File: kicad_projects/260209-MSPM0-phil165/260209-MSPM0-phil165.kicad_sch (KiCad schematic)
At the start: 17 parts, among them J1 USB_C_Receptacle_USB2.0_16P, U1 MSPM0G3507SPTR, U2 USBLC6-2SC6, U3 SPX3819M5-L-3-3, X1 8MHz

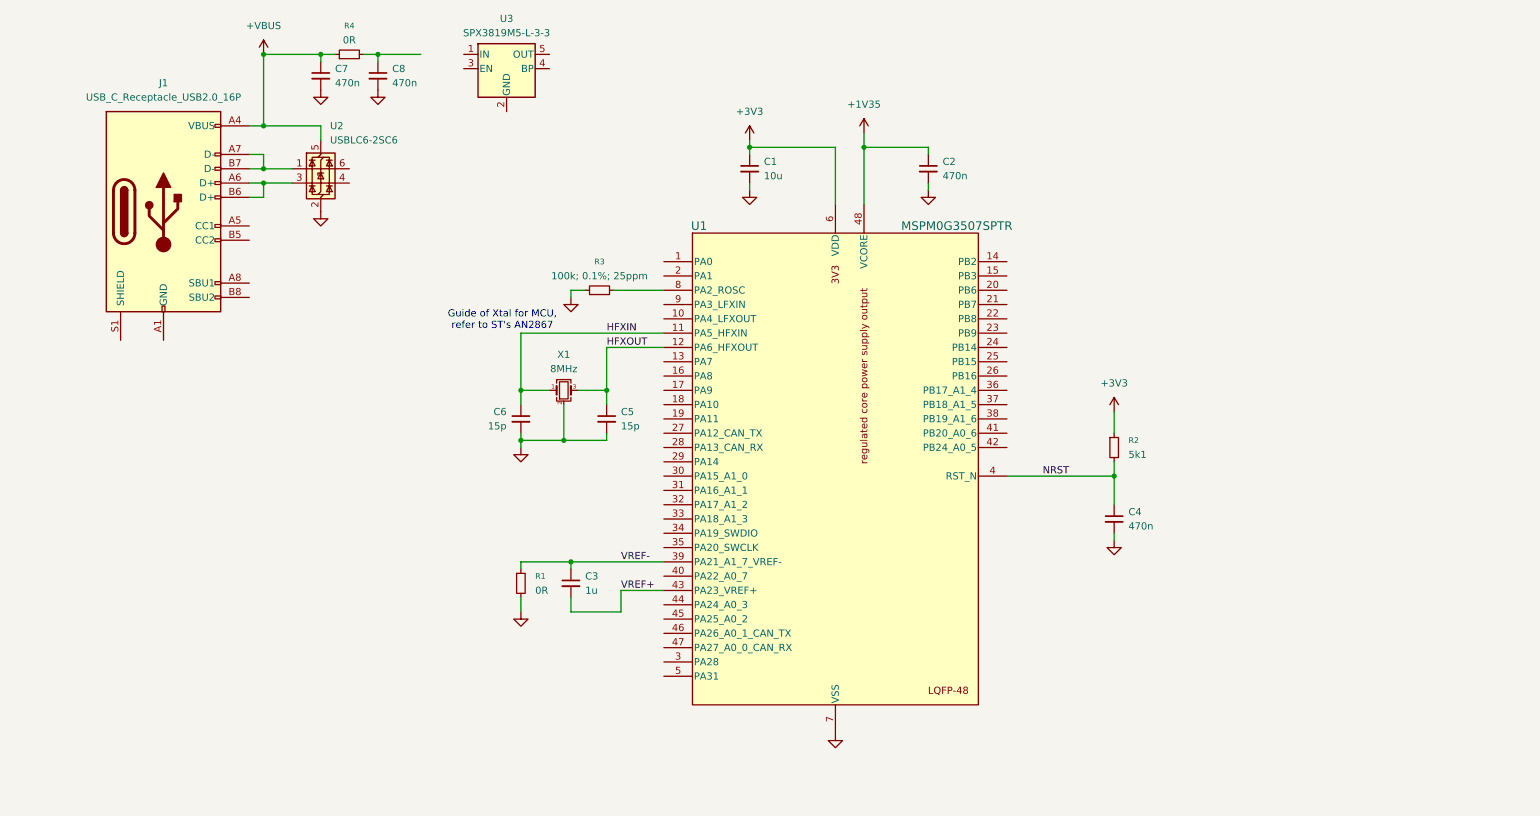
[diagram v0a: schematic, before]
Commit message: regular
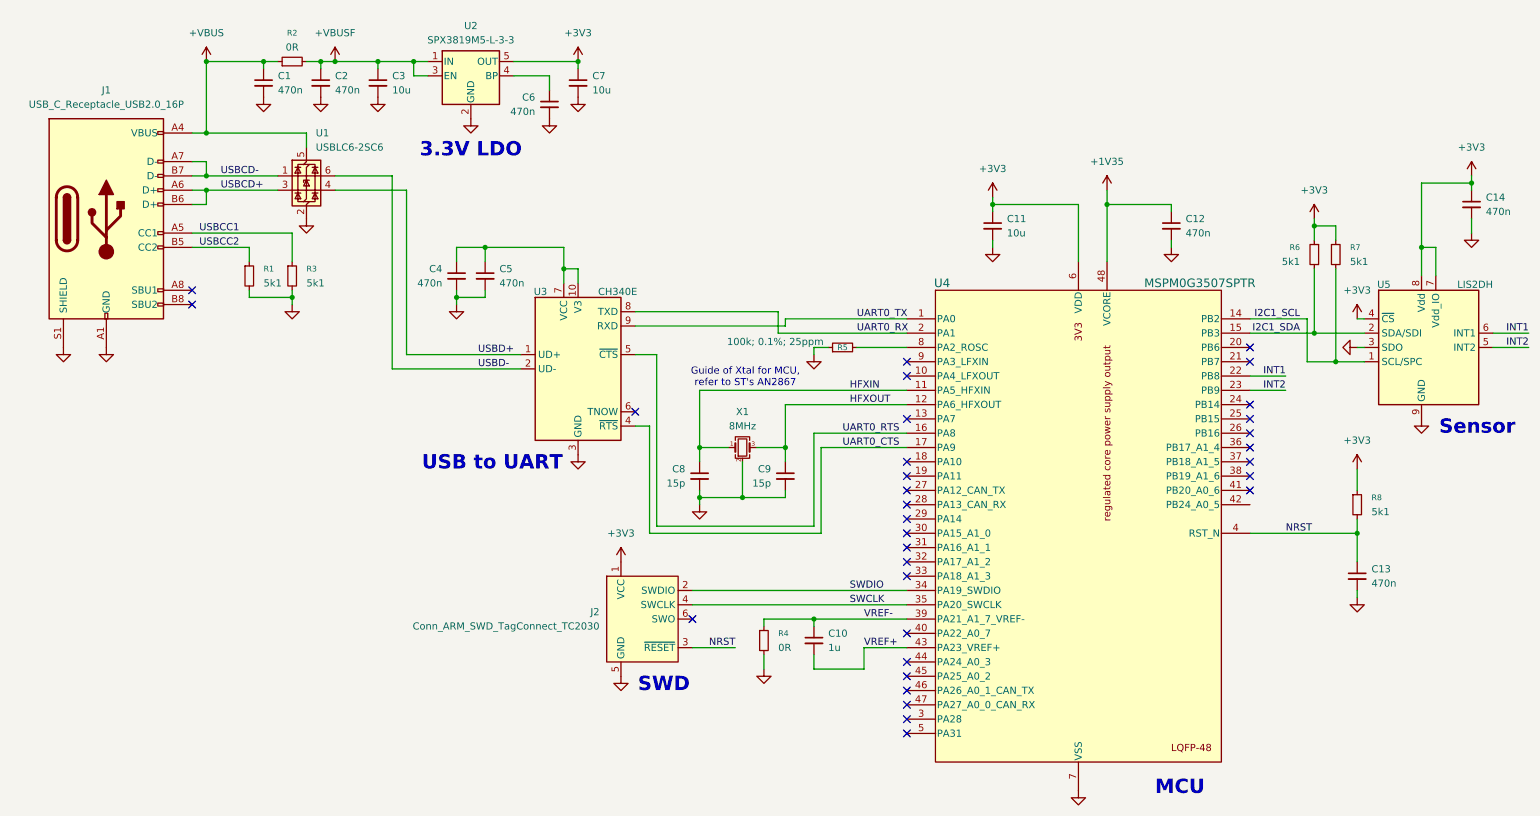
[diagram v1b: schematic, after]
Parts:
- added C14, C4, C5, C6: 470n, Capacitor_SMD:C_0805_2012Metric, symbol Device:C_Small
- added C3, C7: 10u, Capacitor_SMD:C_0805_2012Metric, symbol Device:C_Small
- added J2: Conn_ARM_SWD_TagConnect_TC2030, Connector:Tag-Connect_TC2030-IDC-FP_2x03_P1.27mm_Vertical, symbol Connector:Conn_ARM_SWD_TagConnect_TC2030
- added R1, R3, R6, R7: 5k1, Resistor_SMD:R_0603_1608Metric, symbol Device:R_Small
- added U3: CH340E, Package_SO:MSOP-10_3x3mm_P0.5mm, symbol Interface_USB:CH340E
- added U5: LIS2DH, Package_LGA:LGA-14_2x2mm_P0.35mm_LayoutBorder3x4y, symbol Sensor_Motion:LIS2DH
- renumbered C7 to C1, C3 to C10, C1 to C11, C2 to C12, C4 to C13, C8 to C2, C6 to C8, C5 to C9, R4 to R2, R1 to R4, R3 to R5, R2 to R8, U2 to U1, U3 to U2, U1 to U4
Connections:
- net +3V3: now also U2.5 (OUT), C14.1, C7.1, J2.1 (VCC), R6.1, R7.1, U5.4 (~{CS}), U5.7 (Vdd_IO), U5.8 (Vdd)
- net GND: now also J1.A1 (GND), J1.A12 (GND), J1.B1 (GND), J1.B12 (GND), J1.S1 (SHIELD), U2.2 (GND), C14.2, C3.2, C4.2, C5.2, C6.2, C7.2, J2.5 (GND), R1.2, R3.2, U3.3 (GND), U5.10 (GND), U5.11 (GND), U5.12 (GND), U5.13 (GND), U5.14 (GND), U5.3 (SDO), U5.9 (GND)
- net NRST: now also J2.3 (~{RESET})
- net +VBUSF: now reaches C2.1, R2.2
- net +VBUSF: now also U2.1 (IN), U2.3 (EN), C3.1
- net USBCD-: now reaches J1.A7 (D-), J1.B7 (D-), U1.1 (I/O1)
- net USBCD+: now reaches J1.A6 (D+), J1.B6 (D+), U1.3 (I/O2)
- net USBD+: now reaches U1.4 (I/O2)
- net USBD+: now also U3.1 (UD+)
- net USBD-: now reaches U1.6 (I/O1)
- net USBD-: now also U3.2 (UD-)
- net UART0_TX: now reaches U4.1 (PA0)
- net UART0_TX: now also U3.9 (RXD)
- net I2C1_SCL: now reaches U4.14 (PB2)
- net I2C1_SCL: now also R7.2, U5.1 (SCL/SPC)
- net I2C1_SDA: now reaches U4.15 (PB3)
- net I2C1_SDA: now also R6.2, U5.2 (SDA/SDI)
- net UART0_RTS: now reaches U4.16 (PA8)
- net UART0_RTS: now also U3.5 (~{CTS})
- net UART0_CTS: now reaches U4.17 (PA9)
- net UART0_CTS: now also U3.4 (~{RTS})
- net UART0_RX: now reaches U4.2 (PA1)
- net UART0_RX: now also U3.8 (TXD)
- net INT1: now reaches U4.22 (PB8)
- net INT1: now also U5.6 (INT1)
- net INT2: now reaches U4.23 (PB9)
- net INT2: now also U5.5 (INT2)
- net SWDIO: now reaches U4.34 (PA19_SWDIO)
- net SWDIO: now also J2.2 (SWDIO)
- net SWCLK: now reaches U4.35 (PA20_SWCLK)
- net SWCLK: now also J2.4 (SWCLK)
- net USBCC1: now reaches J1.A5 (CC1)
- net USBCC1: now also R3.1
- net USBCC2: now reaches J1.B5 (CC2)
- net USBCC2: now also R1.1
- net at U2.4 (BP): now also C6.1
- new net: C4.1, C5.1, U3.10 (V3), U3.7 (VCC)
- no-connect marks 0 -> 32
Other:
- note added: "3.3V LDO"
- note added: "MCU"
- note added: "SWD"
- note added: "Sensor"
- note added: "USB to UART"
- moved on the sheet: C1, C10, C11, C12, C13, C2, C8, C9, J1, R2, R4, R5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
